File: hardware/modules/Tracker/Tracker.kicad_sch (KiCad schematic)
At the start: 0 parts

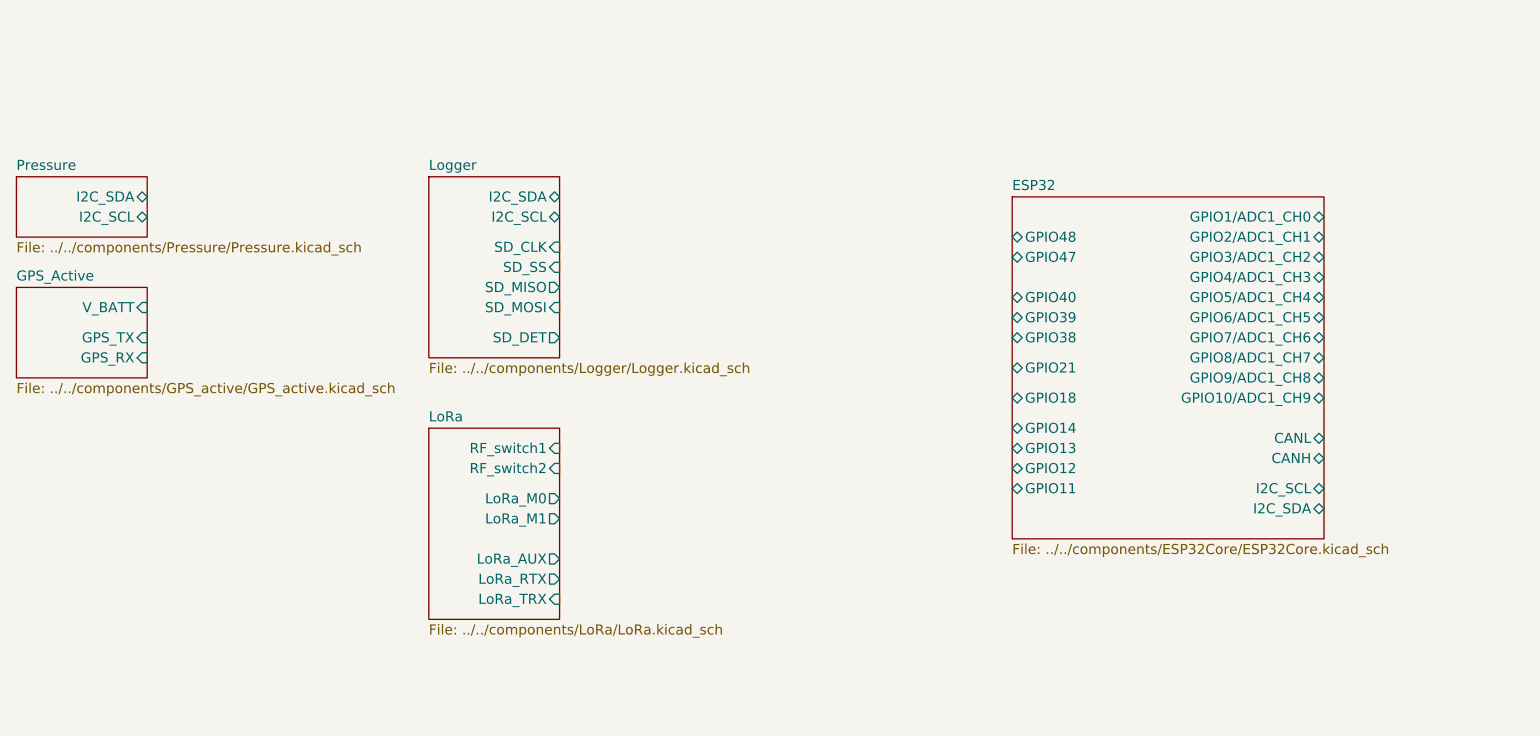
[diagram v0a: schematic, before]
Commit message: 諸々修正しました
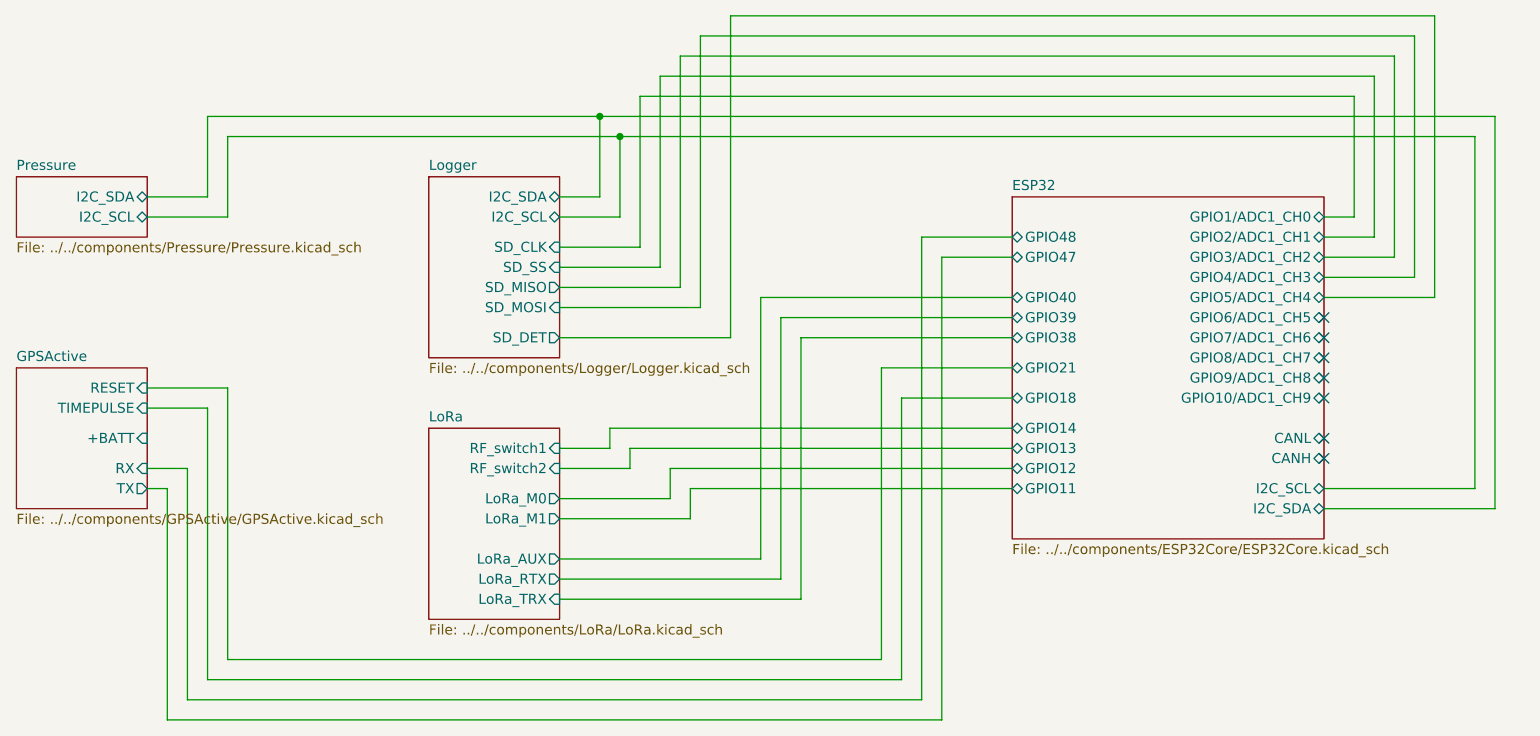
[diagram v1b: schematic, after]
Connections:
- no-connect marks 0 -> 7
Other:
- removed sheet GPS_Active
- added sheet GPSActive (../../components/GPSActive/GPSActive.kicad_sch)
